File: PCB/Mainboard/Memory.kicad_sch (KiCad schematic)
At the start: 5 parts, among them J15 RAM Module, U28 M5M4V16160, U33 M5M4V16160

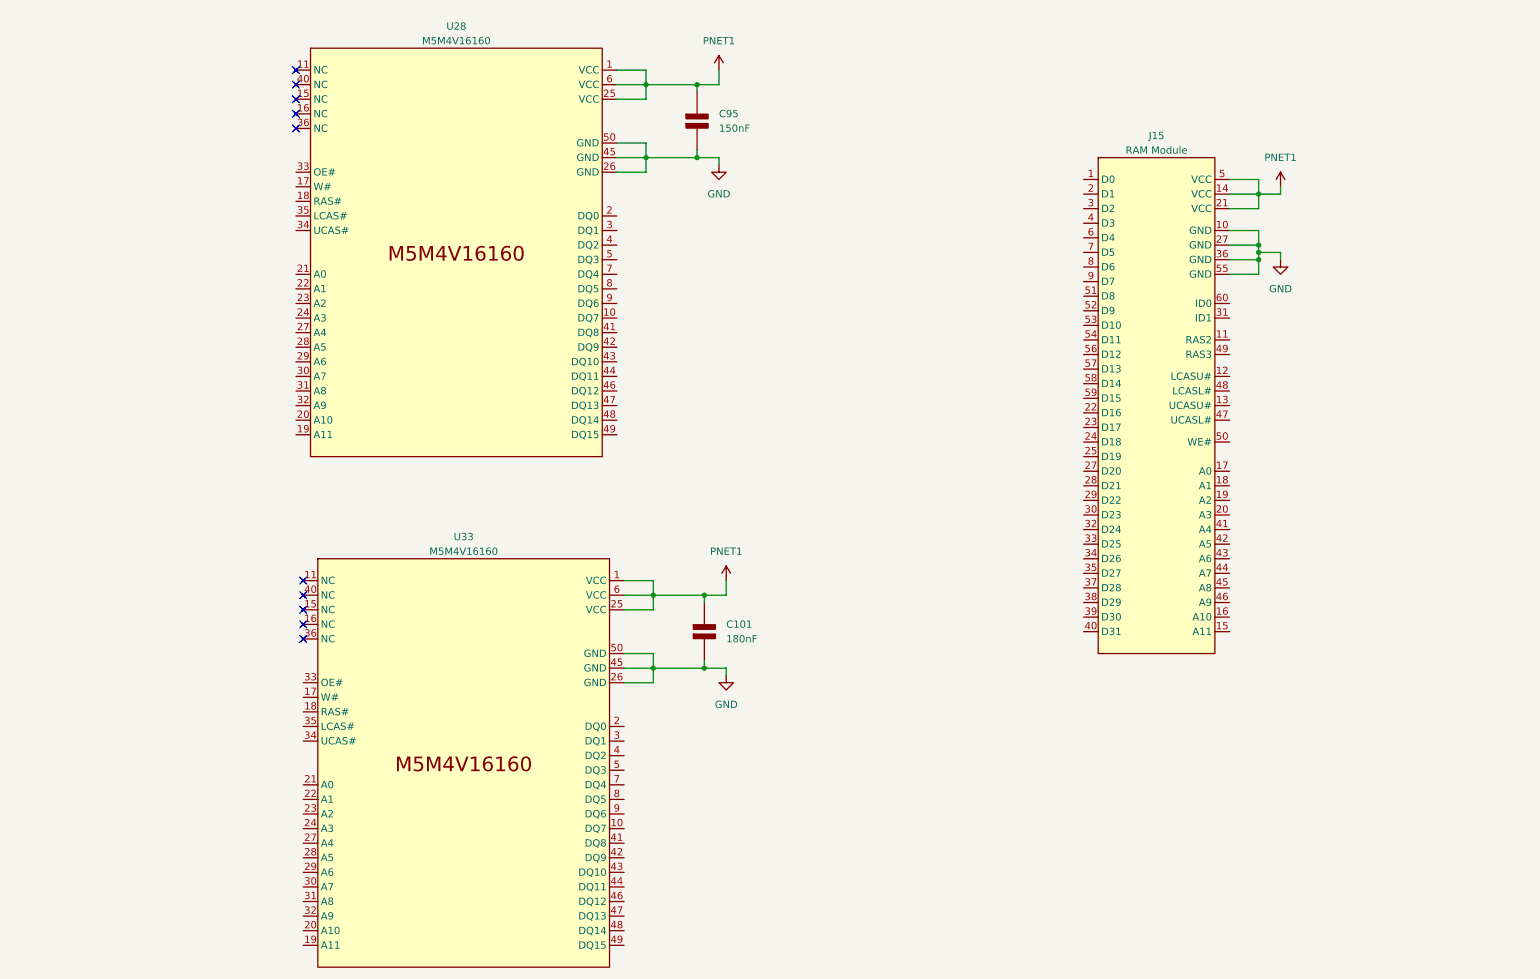
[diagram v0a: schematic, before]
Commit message: Add files via upload
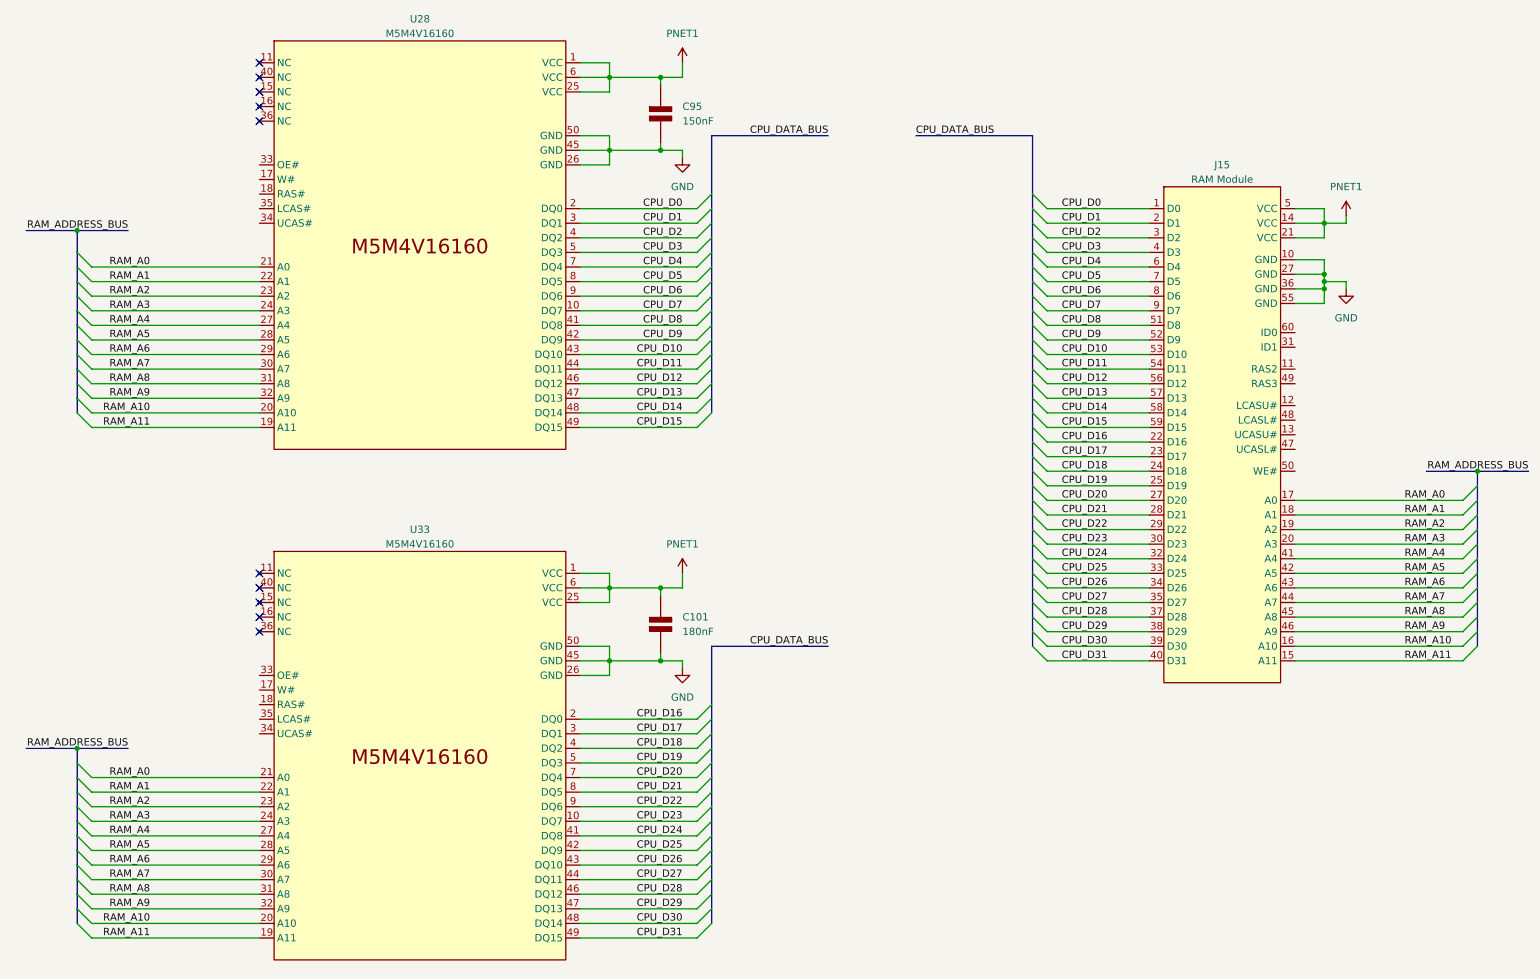
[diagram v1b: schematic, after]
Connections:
- net CPU_D0: now reaches J15.1 (D0)
- net CPU_D0: now also U28.2 (DQ0)
- net RAM_A11: now reaches J15.15 (A11)
- net RAM_A11: now also U28.19 (A11), U33.19 (A11)
- net RAM_A10: now reaches J15.16 (A10)
- net RAM_A10: now also U28.20 (A10), U33.20 (A10)
- net RAM_A0: now reaches J15.17 (A0)
- net RAM_A0: now also U28.21 (A0), U33.21 (A0)
- net RAM_A1: now reaches J15.18 (A1)
- net RAM_A1: now also U28.22 (A1), U33.22 (A1)
- net RAM_A2: now reaches J15.19 (A2)
- net RAM_A2: now also U28.23 (A2), U33.23 (A2)
- net CPU_D1: now reaches J15.2 (D1)
- net CPU_D1: now also U28.3 (DQ1)
- net RAM_A3: now reaches J15.20 (A3)
- net RAM_A3: now also U28.24 (A3), U33.24 (A3)
- net CPU_D16: now reaches J15.22 (D16)
- net CPU_D16: now also U33.2 (DQ0)
- net CPU_D17: now reaches J15.23 (D17)
- net CPU_D17: now also U33.3 (DQ1)
- net CPU_D18: now reaches J15.24 (D18)
- net CPU_D18: now also U33.4 (DQ2)
- net CPU_D19: now reaches J15.25 (D19)
- net CPU_D19: now also U33.5 (DQ3)
- net CPU_D21: now reaches J15.28 (D21)
- net CPU_D21: now also U33.8 (DQ5)
- net CPU_D22: now reaches J15.29 (D22)
- net CPU_D22: now also U33.9 (DQ6)
- net CPU_D2: now reaches J15.3 (D2)
- net CPU_D2: now also U28.4 (DQ2)
- net CPU_D23: now reaches J15.30 (D23)
- net CPU_D23: now also U33.10 (DQ7)
- net CPU_D24: now reaches J15.32 (D24)
- net CPU_D24: now also U33.41 (DQ8)
- net CPU_D25: now reaches J15.33 (D25)
- net CPU_D25: now also U33.42 (DQ9)
- net CPU_D26: now reaches J15.34 (D26)
- net CPU_D26: now also U33.43 (DQ10)
- net CPU_D27: now reaches J15.35 (D27)
- net CPU_D27: now also U33.44 (DQ11)
- net CPU_D28: now reaches J15.37 (D28)
- net CPU_D28: now also U33.46 (DQ12)
- net CPU_D29: now reaches J15.38 (D29)
- net CPU_D29: now also U33.47 (DQ13)
- net CPU_D30: now reaches J15.39 (D30)
- net CPU_D30: now also U33.48 (DQ14)
- net CPU_D3: now reaches J15.4 (D3)
- net CPU_D3: now also U28.5 (DQ3)
- net CPU_D31: now reaches J15.40 (D31)
- net CPU_D31: now also U33.49 (DQ15)
- net RAM_A4: now reaches J15.41 (A4)
- net RAM_A4: now also U28.27 (A4), U33.27 (A4)
- net RAM_A5: now reaches J15.42 (A5)
- net RAM_A5: now also U28.28 (A5), U33.28 (A5)
- net RAM_A6: now reaches J15.43 (A6)
- net RAM_A6: now also U28.29 (A6), U33.29 (A6)
- net RAM_A7: now reaches J15.44 (A7)
- net RAM_A7: now also U28.30 (A7), U33.30 (A7)
- net RAM_A8: now reaches J15.45 (A8)
- net RAM_A8: now also U28.31 (A8), U33.31 (A8)
- net RAM_A9: now reaches J15.46 (A9)
- net RAM_A9: now also U28.32 (A9), U33.32 (A9)
- net CPU_D8: now reaches J15.51 (D8)
- net CPU_D8: now also U28.41 (DQ8)
- net CPU_D9: now reaches J15.52 (D9)
- net CPU_D9: now also U28.42 (DQ9)
- net CPU_D10: now reaches J15.53 (D10)
- net CPU_D10: now also U28.43 (DQ10)
- net CPU_D11: now reaches J15.54 (D11)
- net CPU_D11: now also U28.44 (DQ11)
- net CPU_D12: now reaches J15.56 (D12)
- net CPU_D12: now also U28.46 (DQ12)
- net CPU_D13: now reaches J15.57 (D13)
- net CPU_D13: now also U28.47 (DQ13)
- net CPU_D14: now reaches J15.58 (D14)
- net CPU_D14: now also U28.48 (DQ14)
- net CPU_D15: now reaches J15.59 (D15)
- net CPU_D15: now also U28.49 (DQ15)
- net CPU_D4: now reaches J15.6 (D4)
- net CPU_D4: now also U28.7 (DQ4)
- net CPU_D5: now reaches J15.7 (D5)
- net CPU_D5: now also U28.8 (DQ5)
- net CPU_D6: now reaches J15.8 (D6)
- net CPU_D6: now also U28.9 (DQ6)
- net CPU_D7: now reaches J15.9 (D7)
- net CPU_D7: now also U28.10 (DQ7)
- net CPU_D20: now reaches U33.7 (DQ4)
- net CPU_D20: now also J15.27 (GND)
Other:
- moved on the sheet: C101, C95, J15, U28, U33
